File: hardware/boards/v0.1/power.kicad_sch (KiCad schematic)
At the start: 66 parts, among them IC3 SP3401-02UTG, J2 USB, U20 TPS62A02ADRLR, U23 BQ21040DBV, U30 FUSB307BVMPX, U31 TPS22929D, U32 LTC2942, U36 STM6601GU2BDM6F, U39 TPS61252DSG, U40 MIC2017YM6

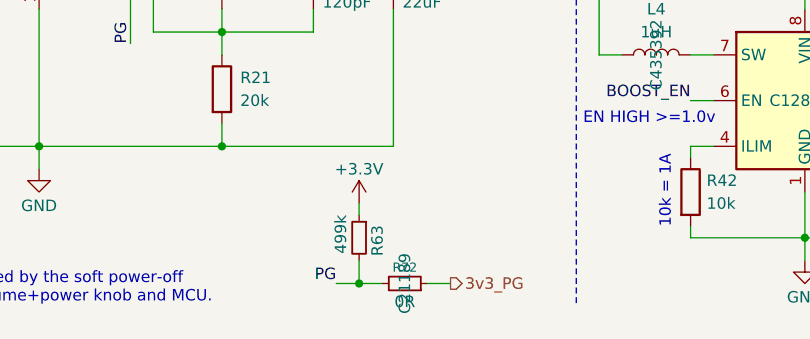
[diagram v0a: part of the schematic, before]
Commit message: chore: schematic cleanup
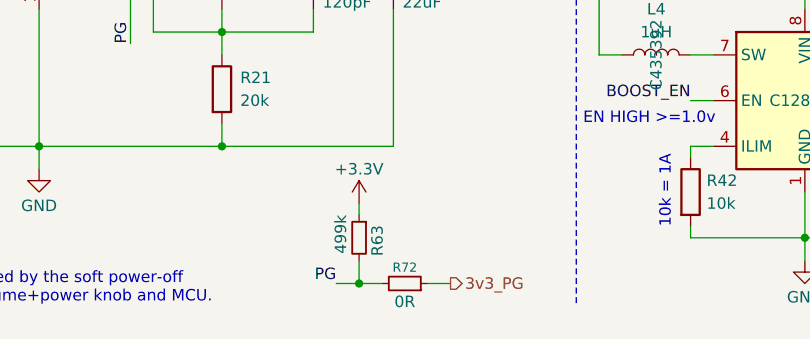
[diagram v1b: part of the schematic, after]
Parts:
- D19: JLC (none) -> C130719
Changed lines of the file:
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@@
 			)
 		)
-		(property "JLC" ""
+		(property "JLC" "C130719"
 			(at 250.19 82.55 0)
 			(effects
@@
 					(size 1.27 1.27)
 				)
+				(hide yes)
 			)
 		)
@@
 				)
 				(justify left)
-			)
-		)
-		(property "MANUFACTURER" ""
-			(at 250.19 82.55 0)
-			(effects
-				(font
-					(size 1.27 1.27)
-				)
-			)
-		)
-		(property "MAXIMUM_PACKAGE_HEIGHT" ""
-			(at 250.19 82.55 0)
-			(effects
-				(font
-					(size 1.27 1.27)
-				)
-			)
-		)
-		(property "Connector" ""
-			(at 250.19 82.55 0)
-			(effects
-				(font
-					(size 1.27 1.27)
-				)
 			)
 		)
@@
 					(size 1.27 1.27)
 				)
-			)
-		)
+				(hide yes)
+			)
+		)
